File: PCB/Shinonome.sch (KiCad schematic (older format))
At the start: 41 parts, among them J1 MJ-4PP-9, SW1 SW_PUSH, SW10 SW_PUSH, SW11 SW_PUSH, SW12 SW_PUSH, SW13 SW_PUSH, SW14 SW_PUSH, SW15 SW_PUSH, SW16 SW_PUSH, SW17 SW_PUSH, SW18 SW_PUSH, SW19 SW_PUSH, SW2 SW_PUSH, SW20 reset, SW3 SW_PUSH, SW4 SW_PUSH, SW5 SW_PUSH, SW6 SW_PUSH, SW7 SW_PUSH, SW8 SW_PUSH, SW9 SW_PUSH, U1 ProMicro

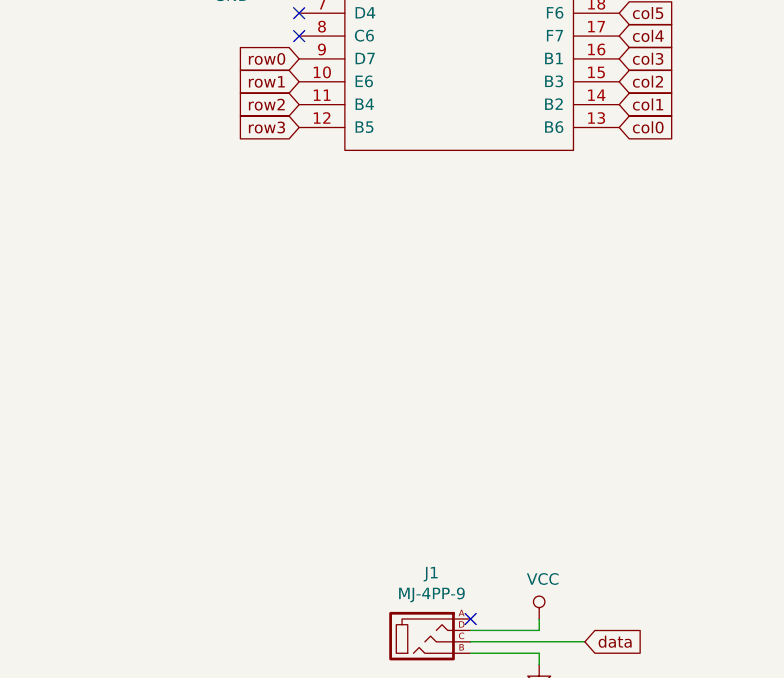
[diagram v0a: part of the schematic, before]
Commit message: first pass pcb complete
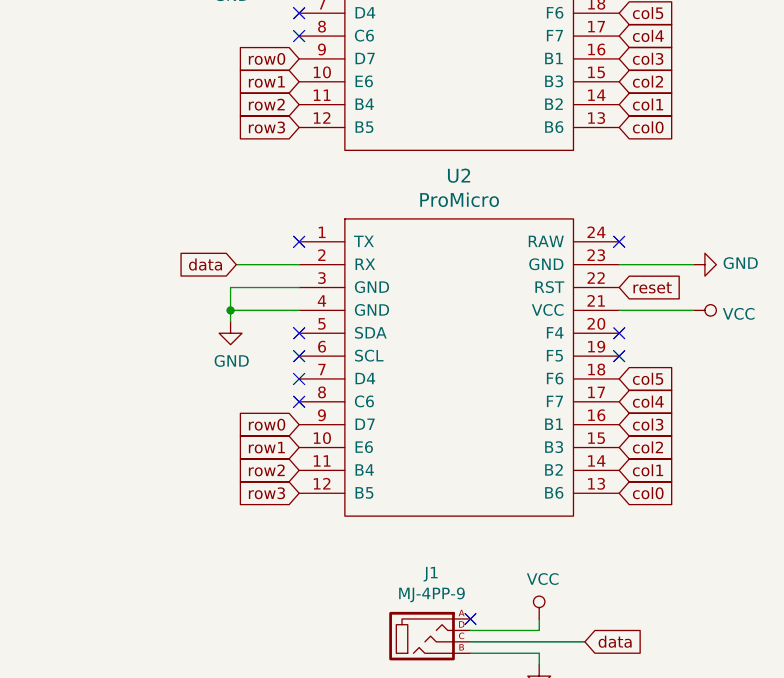
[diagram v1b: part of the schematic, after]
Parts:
- added U2: ProMicro, kbd:ProMicro_v2_Backside, symbol kbd:ProMicro
- SW1, SW10, SW11, SW12, SW13, SW14, SW15, SW16, SW17, SW18, SW19, SW2, SW3, SW4, SW5, SW6, SW7, SW8, SW9: footprint kbd:CherryMX_Hotswap -> helix:MX_ALPS_PG1350_noLed
- U1: footprint kbd:ProMicro_v2 -> kbd:ProMicro_v2_Backside
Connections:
- net GND: now also U2.23 (GND), U2.3 (GND), U2.4 (GND)
- net VCC: now also U2.21 (VCC)
- net col0: now also U2.13 (B6)
- net col1: now also U2.14 (B2)
- net col2: now also U2.15 (B3)
- net col3: now also U2.16 (B1)
- net col4: now also U2.17 (F7)
- net col5: now also U2.18 (F6)
- net data: now also U2.2 (RX)
- net reset: now also U2.22 (RST)
- net row0: now also U2.9 (D7)
- net row1: now also U2.10 (E6)
- net row2: now also U2.11 (B4)
- net row3: now also U2.12 (B5)
- no-connect marks 9 -> 17
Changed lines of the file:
@@
 EESchema Schematic File Version 4
+LIBS:Shinonome-cache
 EELAYER 26 0
 EELAYER END
@@
 F 0 "U1" H 9550 3087 60  0000 C CNN
 F 1 "ProMicro" H 9550 2981 60  0000 C CNN
-F 2 "kbd:ProMicro_v2" H 9650 1000 60  0001 C CNN
+F 2 "kbd:ProMicro_v2_Backside" H 9650 1000 60  0001 C CNN
 F 3 "" H 9650 1000 60  0000 C CNN
 	1    9550 2050
@@
 F 0 "SW1" H 1750 1955 50  0000 C CNN
 F 1 "SW_PUSH" H 1750 1864 50  0000 C CNN
-F 2 "kbd:CherryMX_Hotswap" H 1750 1700 50  0001 C CNN
+F 2 "helix:MX_ALPS_PG1350_noLed" H 1750 1700 50  0001 C CNN
 F 3 "" H 1750 1700 50  0000 C CNN
 	1    1750 1700
@@
 F 0 "SW4" H 2650 1955 50  0000 C CNN
 F 1 "SW_PUSH" H 2650 1864 50  0000 C CNN
-F 2 "kbd:CherryMX_Hotswap" H 2650 1700 50  0001 C CNN
+F 2 "helix:MX_ALPS_PG1350_noLed" H 2650 1700 50  0001 C CNN
 F 3 "" H 2650 1700 50  0000 C CNN
 	1    2650 1700
@@
 F 0 "SW7" H 3550 1955 50  0000 C CNN
 F 1 "SW_PUSH" H 3550 1864 50  0000 C CNN
-F 2 "kbd:CherryMX_Hotswap" H 3550 1700 50  0001 C CNN
+F 2 "helix:MX_ALPS_PG1350_noLed" H 3550 1700 50  0001 C CNN
 F 3 "" H 3550 1700 50  0000 C CNN
 	1    3550 1700
@@
 F 0 "SW10" H 4450 1955 50  0000 C CNN
 F 1 "SW_PUSH" H 4450 1864 50  0000 C CNN
-F 2 "kbd:CherryMX_Hotswap" H 4450 1700 50  0001 C CNN
+F 2 "helix:MX_ALPS_PG1350_noLed" H 4450 1700 50  0001 C CNN
 F 3 "" H 4450 1700 50  0000 C CNN
 	1    4450 1700
@@
 F 0 "SW14" H 5350 1955 50  0000 C CNN
 F 1 "SW_PUSH" H 5350 1864 50  0000 C CNN
-F 2 "kbd:CherryMX_Hotswap" H 5350 1700 50  0001 C CNN
+F 2 "helix:MX_ALPS_PG1350_noLed" H 5350 1700 50  0001 C CNN
 F 3 "" H 5350 1700 50  0000 C CNN
 	1    5350 1700
@@
 F 0 "SW2" H 1750 2605 50  0000 C CNN
 F 1 "SW_PUSH" H 1750 2514 50  0000 C CNN
-F 2 "kbd:CherryMX_Hotswap" H 1750 2350 50  0001 C CNN
+F 2 "helix:MX_ALPS_PG1350_noLed" H 1750 2350 50  0001 C CNN
 F 3 "" H 1750 2350 50  0000 C CNN
 	1    1750 2350
@@
 F 0 "SW5" H 2650 2605 50  0000 C CNN
 F 1 "SW_PUSH" H 2650 2514 50  0000 C CNN
-F 2 "kbd:CherryMX_Hotswap" H 2650 2350 50  0001 C CNN
+F 2 "helix:MX_ALPS_PG1350_noLed" H 2650 2350 50  0001 C CNN
 F 3 "" H 2650 2350 50  0000 C CNN
 	1    2650 2350
@@
 F 0 "SW8" H 3550 2605 50  0000 C CNN
 F 1 "SW_PUSH" H 3550 2514 50  0000 C CNN
-F 2 "kbd:CherryMX_Hotswap" H 3550 2350 50  0001 C CNN
+F 2 "helix:MX_ALPS_PG1350_noLed" H 3550 2350 50  0001 C CNN
 F 3 "" H 3550 2350 50  0000 C CNN
 	1    3550 2350
@@
 F 0 "SW11" H 4450 2605 50  0000 C CNN
 F 1 "SW_PUSH" H 4450 2514 50  0000 C CNN
-F 2 "kbd:CherryMX_Hotswap" H 4450 2350 50  0001 C CNN
+F 2 "helix:MX_ALPS_PG1350_noLed" H 4450 2350 50  0001 C CNN
 F 3 "" H 4450 2350 50  0000 C CNN
 	1    4450 2350
@@
 F 0 "SW15" H 5350 2605 50  0000 C CNN
 F 1 "SW_PUSH" H 5350 2514 50  0000 C CNN
-F 2 "kbd:CherryMX_Hotswap" H 5350 2350 50  0001 C CNN
+F 2 "helix:MX_ALPS_PG1350_noLed" H 5350 2350 50  0001 C CNN
 F 3 "" H 5350 2350 50  0000 C CNN
 	1    5350 2350
@@
 F 0 "SW3" H 1750 3255 50  0000 C CNN
 F 1 "SW_PUSH" H 1750 3164 50  0000 C CNN
-F 2 "kbd:CherryMX_Hotswap" H 1750 3000 50  0001 C CNN
+F 2 "helix:MX_ALPS_PG1350_noLed" H 1750 3000 50  0001 C CNN
 F 3 "" H 1750 3000 50  0000 C CNN
 	1    1750 3000
@@
 F 0 "SW6" H 2650 3255 50  0000 C CNN
 F 1 "SW_PUSH" H 2650 3164 50  0000 C CNN
-F 2 "kbd:CherryMX_Hotswap" H 2650 3000 50  0001 C CNN
+F 2 "helix:MX_ALPS_PG1350_noLed" H 2650 3000 50  0001 C CNN
 F 3 "" H 2650 3000 50  0000 C CNN
 	1    2650 3000
@@
 F 0 "SW9" H 3550 3255 50  0000 C CNN
 F 1 "SW_PUSH" H 3550 3164 50  0000 C CNN
-F 2 "kbd:CherryMX_Hotswap" H 3550 3000 50  0001 C CNN
+F 2 "helix:MX_ALPS_PG1350_noLed" H 3550 3000 50  0001 C CNN
 F 3 "" H 3550 3000 50  0000 C CNN
 	1    3550 3000
@@
 F 0 "SW12" H 4450 3255 50  0000 C CNN
 F 1 "SW_PUSH" H 4450 3164 50  0000 C CNN
-F 2 "kbd:CherryMX_Hotswap" H 4450 3000 50  0001 C CNN
+F 2 "helix:MX_ALPS_PG1350_noLed" H 4450 3000 50  0001 C CNN
 F 3 "" H 4450 3000 50  0000 C CNN
 	1    4450 3000
@@
 F 0 "SW16" H 5350 3255 50  0000 C CNN
 F 1 "SW_PUSH" H 5350 3164 50  0000 C CNN
-F 2 "kbd:CherryMX_Hotswap" H 5350 3000 50  0001 C CNN
+F 2 "helix:MX_ALPS_PG1350_noLed" H 5350 3000 50  0001 C CNN
 F 3 "" H 5350 3000 50  0000 C CNN
 	1    5350 3000
@@
 F 0 "SW13" H 4450 3905 50  0000 C CNN
 F 1 "SW_PUSH" H 4450 3814 50  0000 C CNN
-F 2 "kbd:CherryMX_Hotswap" H 4450 3650 50  0001 C CNN
+F 2 "helix:MX_ALPS_PG1350_noLed" H 4450 3650 50  0001 C CNN
 F 3 "" H 4450 3650 50  0000 C CNN
 	1    4450 3650
@@
 F 0 "SW17" H 5350 3905 50  0000 C CNN
 F 1 "SW_PUSH" H 5350 3814 50  0000 C CNN
-F 2 "kbd:CherryMX_Hotswap" H 5350 3650 50  0001 C CNN
+F 2 "helix:MX_ALPS_PG1350_noLed" H 5350 3650 50  0001 C CNN
 F 3 "" H 5350 3650 50  0000 C CNN
 	1    5350 3650
@@
 F 0 "SW18" H 6250 3255 50  0000 C CNN
 F 1 "SW_PUSH" H 6250 3164 50  0000 C CNN
-F 2 "kbd:CherryMX_Hotswap" H 6250 3000 50  0001 C CNN
+F 2 "helix:MX_ALPS_PG1350_noLed" H 6250 3000 50  0001 C CNN
 F 3 "" H 6250 3000 50  0000 C CNN
 	1    6250 3000
@@
 F 0 "SW19" H 6250 3905 50  0000 C CNN
 F 1 "SW_PUSH" H 6250 3814 50  0000 C CNN
-F 2 "kbd:CherryMX_Hotswap" H 6250 3650 50  0001 C CNN
+F 2 "helix:MX_ALPS_PG1350_noLed" H 6250 3650 50  0001 C CNN
 F 3 "" H 6250 3650 50  0000 C CNN
 	1    6250 3650
@@
 	1    0    0    -1
 $EndComp
+$Comp
+L kbd:ProMicro U2
+U 1 1 5C5884A0
+P 9550 3650
+F 0 "U2" H 9550 4687 60  0000 C CNN
+F 1 "ProMicro" H 9550 4581 60  0000 C CNN
+F 2 "kbd:ProMicro_v2_Backside" H 9650 2600 60  0001 C CNN
+F 3 "" H 9650 2600 60  0000 C CNN
+	1    9550 3650
+	1    0    0    -1
+$EndComp
+$Comp
+L power:GND #PWR08
+U 1 1 5C5884A7
+P 10575 3000
+F 0 "#PWR08" H 10575 2750 50  0001 C CNN
+F 1 "GND" V 10580 2872 50  0000 R CNN
+F 2 "" H 10575 3000 50  0001 C CNN
+F 3 "" H 10575 3000 50  0001 C CNN
+	1    10575 3000
+	0    -1   -1   0
+$EndComp
+$Comp
+L power:VCC #PWR09
+U 1 1 5C5884AD
+P 10575 3200
+F 0 "#PWR09" H 10575 3050 50  0001 C CNN
+F 1 "VCC" V 10592 3328 50  0000 L CNN
+F 2 "" H 10575 3200 50  0001 C CNN
+F 3 "" H 10575 3200 50  0001 C CNN
+	1    10575 3200
+	0    1    1    0
+$EndComp
+$Comp
+L power:GND #PWR07
+U 1 1 5C5884B3
+P 8550 3250
+F 0 "#PWR07" H 8550 3000 50  0001 C CNN
+F 1 "GND" H 8555 3077 50  0000 C CNN
+F 2 "" H 8550 3250 50  0001 C CNN
+F 3 "" H 8550 3250 50  0001 C CNN
+	1    8550 3250
+	1    0    0    -1
+$EndComp
+Wire Wire Line
+	8850 3100 8550 3100
+Wire Wire Line
+	10250 3000 10575 3000
+Wire Wire Line
+	10250 3200 10575 3200
+Text GLabel 8575 3000 0    50   Input ~ 0
+data
+Wire Wire Line
+	8575 3000 8850 3000
+Text GLabel 10250 3100 2    50   Input ~ 0
+reset
+Text GLabel 8850 3700 0    50   Input ~ 0
+row0
+Text GLabel 8850 3800 0    50   Input ~ 0
+row1
+Text GLabel 8850 3900 0    50   Input ~ 0
+row2
+Text GLabel 8850 4000 0    50   Input ~ 0
+row3
+Text GLabel 10250 4000 2    50   Input ~ 0
+col0
+Text GLabel 10250 3900 2    50   Input ~ 0
+col1
+Text GLabel 10250 3800 2    50   Input ~ 0
+col2
+Text GLabel 10250 3700 2    50   Input ~ 0
+col3
+Text GLabel 10250 3600 2    50   Input ~ 0
+col4
+Text GLabel 10250 3500 2    50   Input ~ 0
+col5
+NoConn ~ 10250 3400
+NoConn ~ 10250 3300
+NoConn ~ 10250 2900
+NoConn ~ 8850 2900
+NoConn ~ 8850 3600
+NoConn ~ 8850 3500
+NoConn ~ 8850 3400
+NoConn ~ 8850 3300
+Wire Wire Line
+	8550 3100 8550 3200
+Wire Wire Line
+	8850 3200 8550 3200
+Connection ~ 8550 3200
+Wire Wire Line
+	8550 3200 8550 3250
 $EndSCHEMATC
